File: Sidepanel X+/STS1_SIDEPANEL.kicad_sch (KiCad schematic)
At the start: 6 parts, among them J1 ZF5S-08-01-T-WT

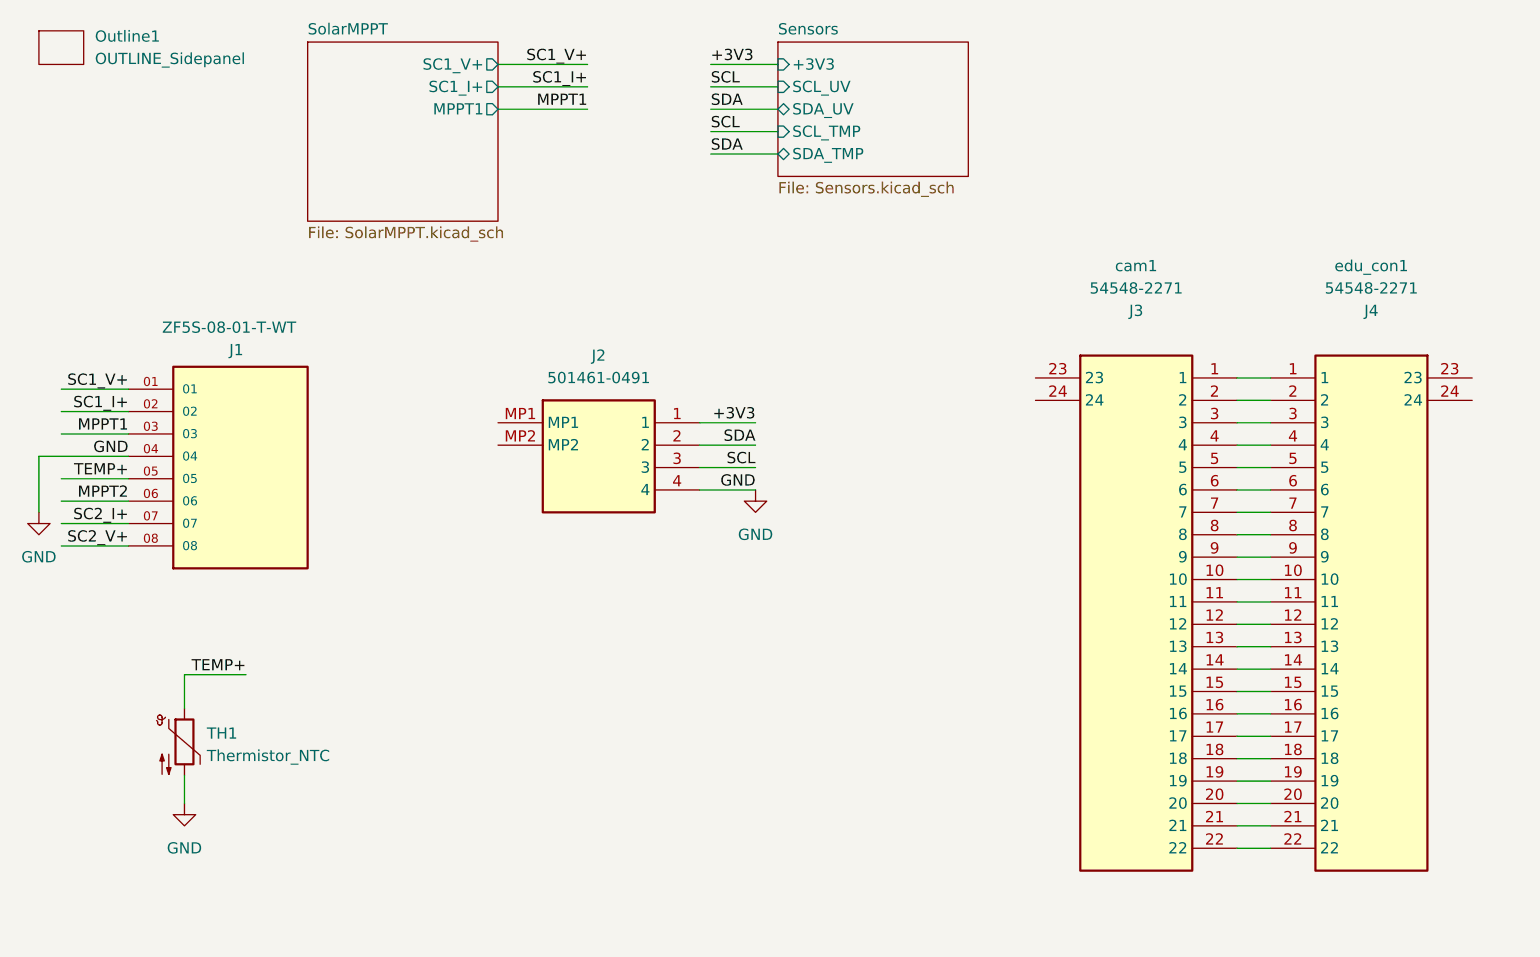
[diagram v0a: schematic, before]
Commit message: small adjustments
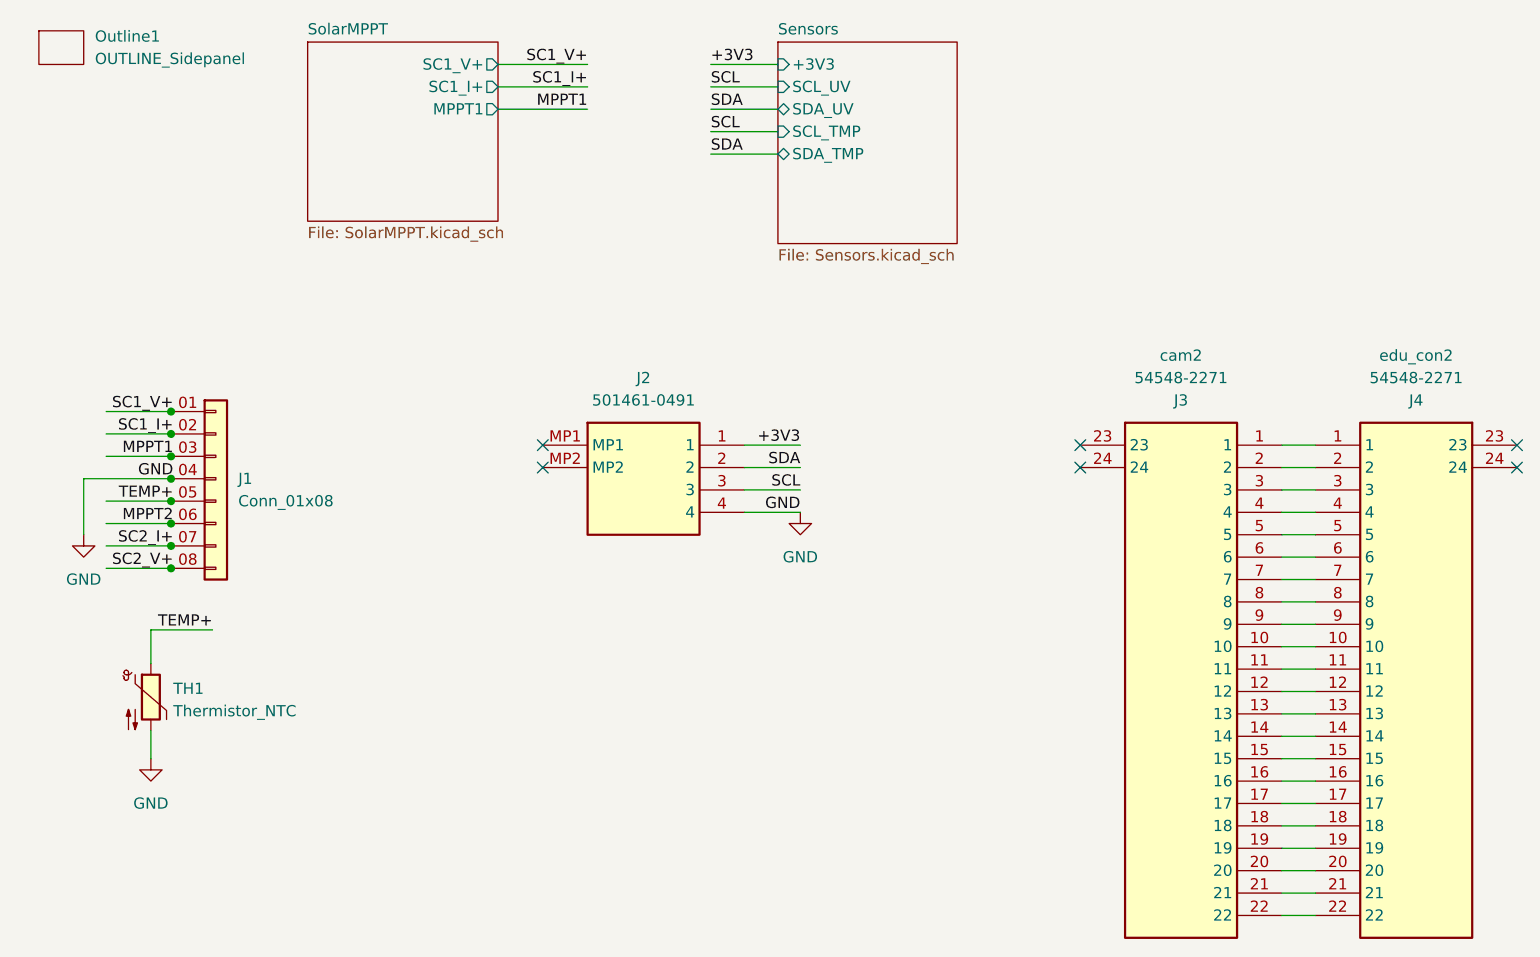
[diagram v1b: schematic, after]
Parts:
- removed J1: ZF5S-08-01-T-WT, Sts:SAMTEC_ZF5S-08-01-T-WT, symbol EPS connector:ZF5S-08-01-T-WT
- removed cam1, edu_con1: 54548-2271, Sts:545482271, symbol Cam:54548-2271
- added J1: Conn_01x08, STS_connector:SAMTEC_ZF5S-08-01-T-WT, symbol Connector_Generic:Conn_01x08
- added cam2, edu_con2: 54548-2271, STS_connector:545482271, symbol Cam:54548-2271
- Outline1: footprint USER_OUTLINE:OUTLINE_SidepanelX+ -> USER_OUTLINE:OUTLINE_SidepanelX-
- UV1: footprint Sts:5014610491 -> STS_connector:5014610491
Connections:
- net GND: now also J1.04 (Pin_4)
- net MPPT1: now also J1.03 (Pin_3)
- net MPPT2: now also J1.06 (Pin_6)
- net SC1_I+: now also J1.02 (Pin_2)
- net SC1_V+: now also J1.01 (Pin_1)
- net SC2_I+: now also J1.07 (Pin_7)
- net SC2_V+: now also J1.08 (Pin_8)
- net TEMP+: now also J1.05 (Pin_5)
- new net: cam2.1, edu_con2.1
- new net: cam2.10, edu_con2.10
- new net: cam2.11, edu_con2.11
- new net: cam2.12, edu_con2.12
- new net: cam2.13, edu_con2.13
- new net: cam2.14, edu_con2.14
- new net: cam2.15, edu_con2.15
- new net: cam2.16, edu_con2.16
- new net: cam2.17, edu_con2.17
- new net: cam2.18, edu_con2.18
- new net: cam2.19, edu_con2.19
- new net: cam2.2, edu_con2.2
- new net: cam2.20, edu_con2.20
- new net: cam2.21, edu_con2.21
- new net: cam2.22, edu_con2.22
- new net: cam2.3, edu_con2.3
- new net: cam2.4, edu_con2.4
- new net: cam2.5, edu_con2.5
- new net: cam2.6, edu_con2.6
- new net: cam2.7, edu_con2.7
- new net: cam2.8, edu_con2.8
- new net: cam2.9, edu_con2.9
- no-connect marks 0 -> 6
